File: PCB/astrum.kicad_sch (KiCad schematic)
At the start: 59 parts, among them J1 USB_C_Receptacle_USB2.0_16P, J10 Conn_01x05_Pin, J11 Screw_Terminal_01x02, J2 Micro_SD_Card, J3 Screw_Terminal_01x02, J5 Conn_01x04_MountingPin, J6 Conn_01x04_MountingPin, J7 Conn_01x10_Pin, J8 Conn_01x10_Pin, J9 Conn_01x05_Pin, SW1 TS-1088-AR02016, SW2 TS-1088-AR02016, U1 STM32H523CEUx, U10 BSS138DW-7-F, U11 LD39015M18R, U2 LDL212PV33R, U3 USBLC6-2SC6, U4 W25Q32JVSS, U6 LSM6DSR, U7 BSS138DW-7-F, U8 DRV8871DDA, U9 DRV8871DDA, Y2 25mHz

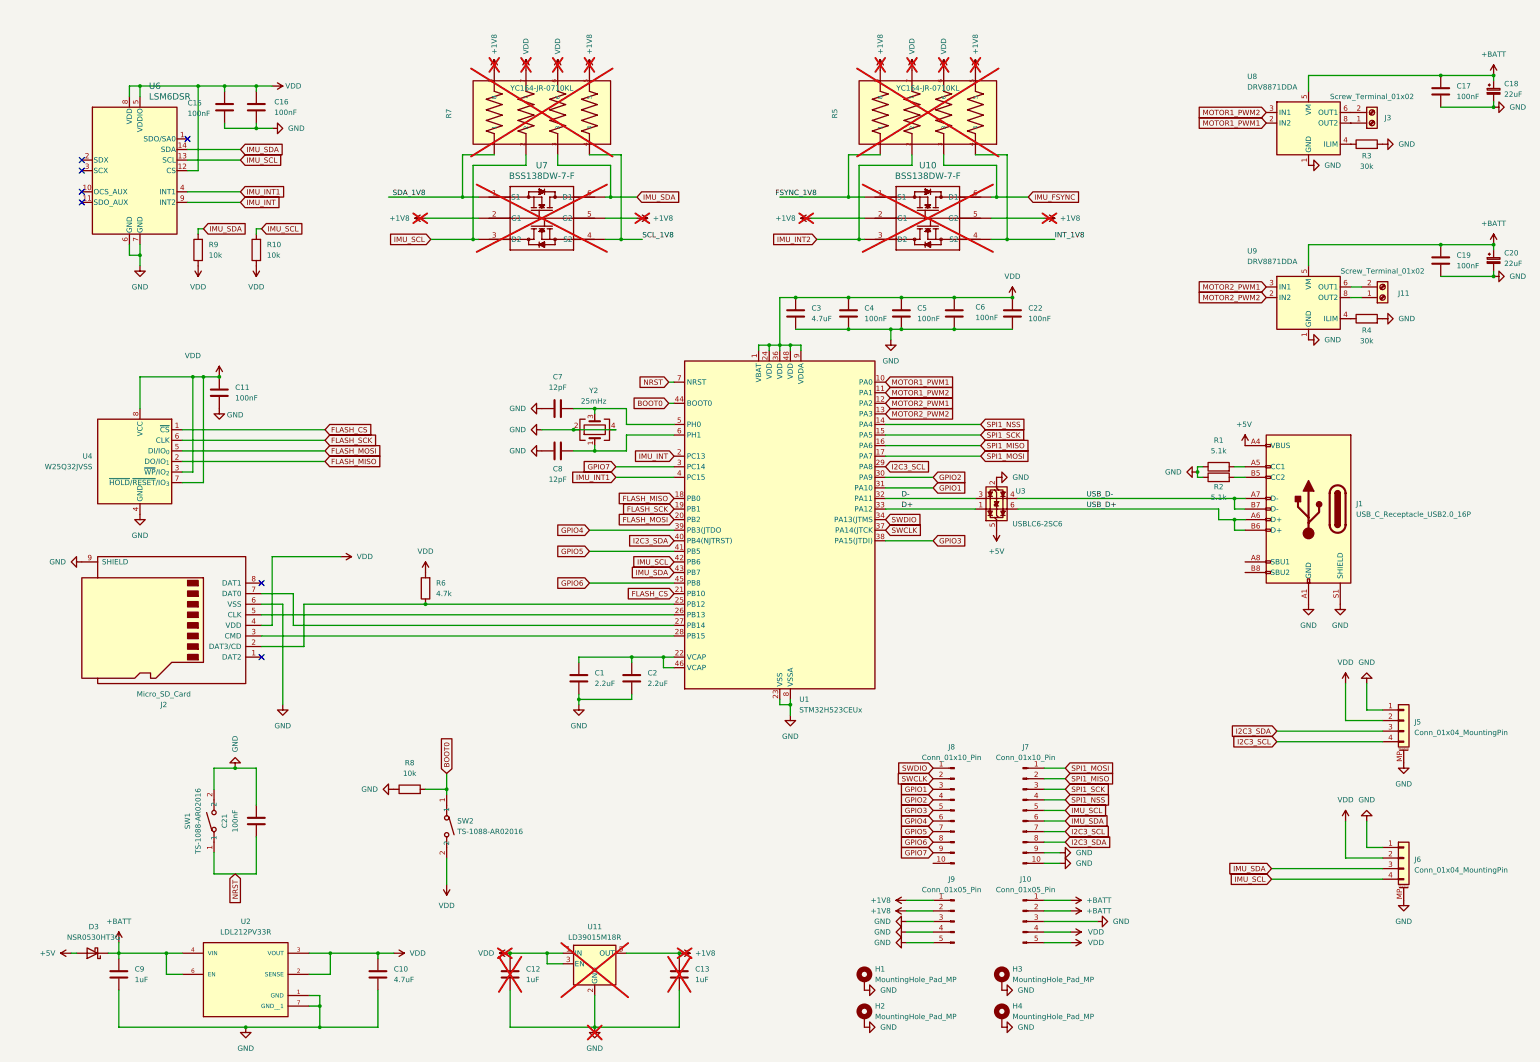
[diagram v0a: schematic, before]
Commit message: update stuff again
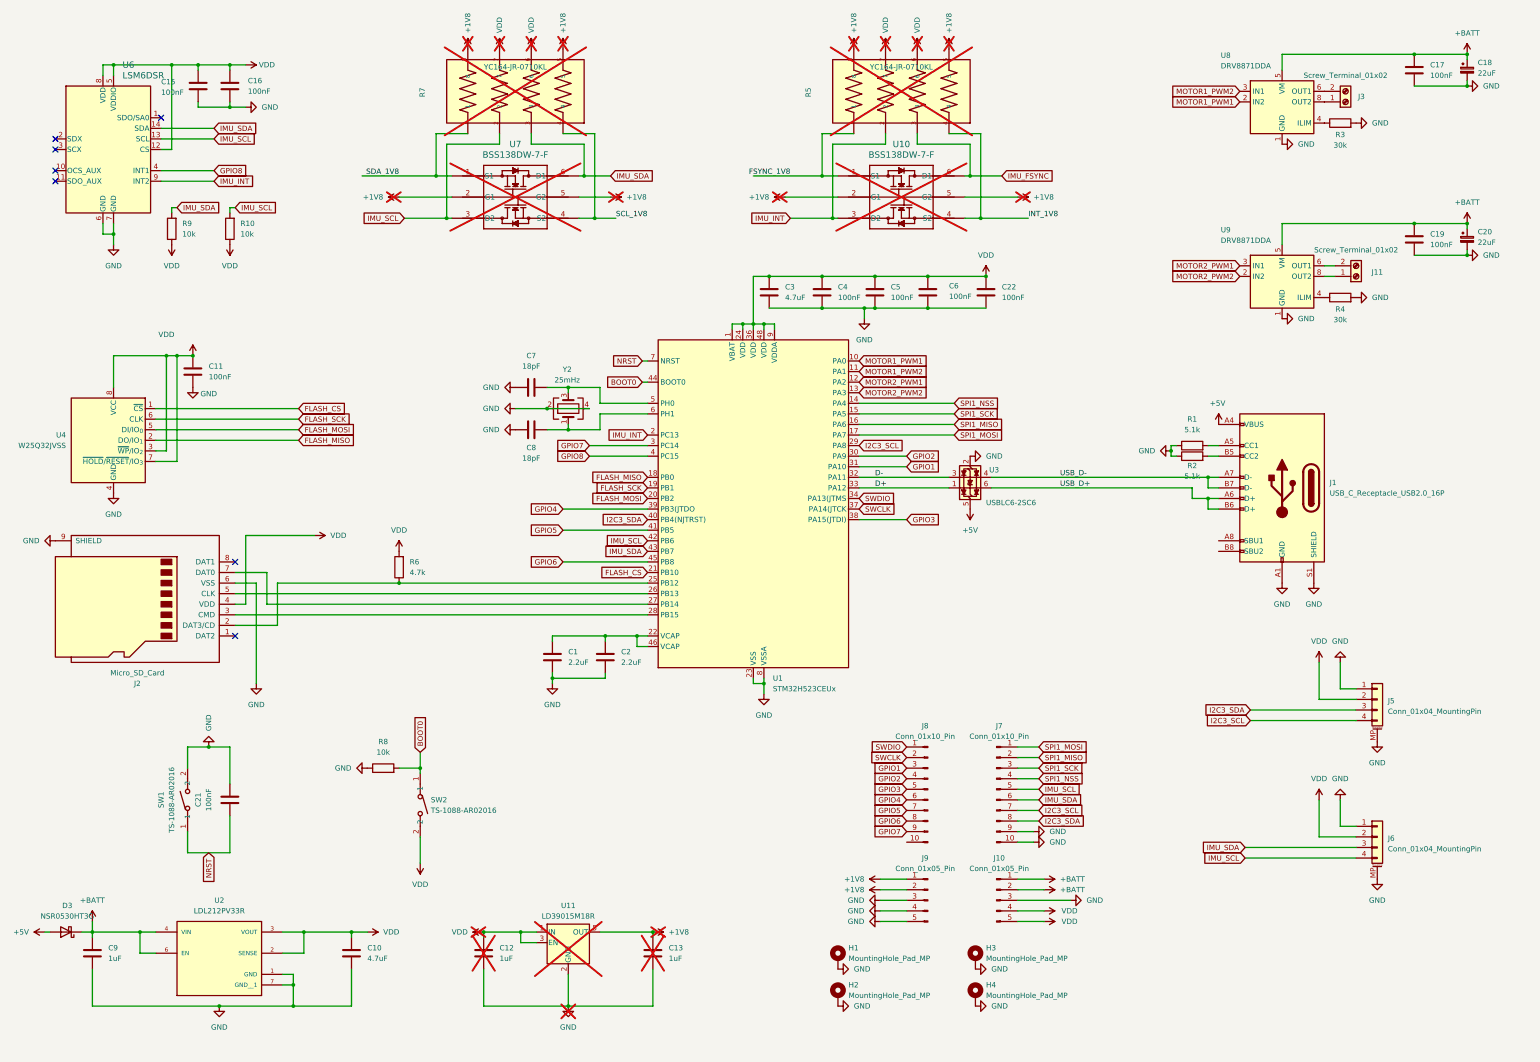
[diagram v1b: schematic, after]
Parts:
- C7, C8: value 12pF -> 18pF
- U6: footprint LSM6DSR:LGA_M6DSR_STM -> LGA_M6DSR_STM
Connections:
- net IMU_INT2 is gone; now on net IMU_INT: R5.2, U10.3 (D2)
- net IMU_INT1 renamed GPIO8
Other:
- moved on the sheet: C1, C10, C11, C12, C13, C15, C16, C17, C18, C19, C2, C20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
